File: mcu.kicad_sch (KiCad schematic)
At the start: 41 parts, among them J1 GPIO, J2 3v3/GND, Q1 MMBTA42, U1 STM32F103C8Tx, X1 SPI_DBG, X2 MTRBTN, X3 Bluetooth, X4 Buzzer, Y1 8MHz

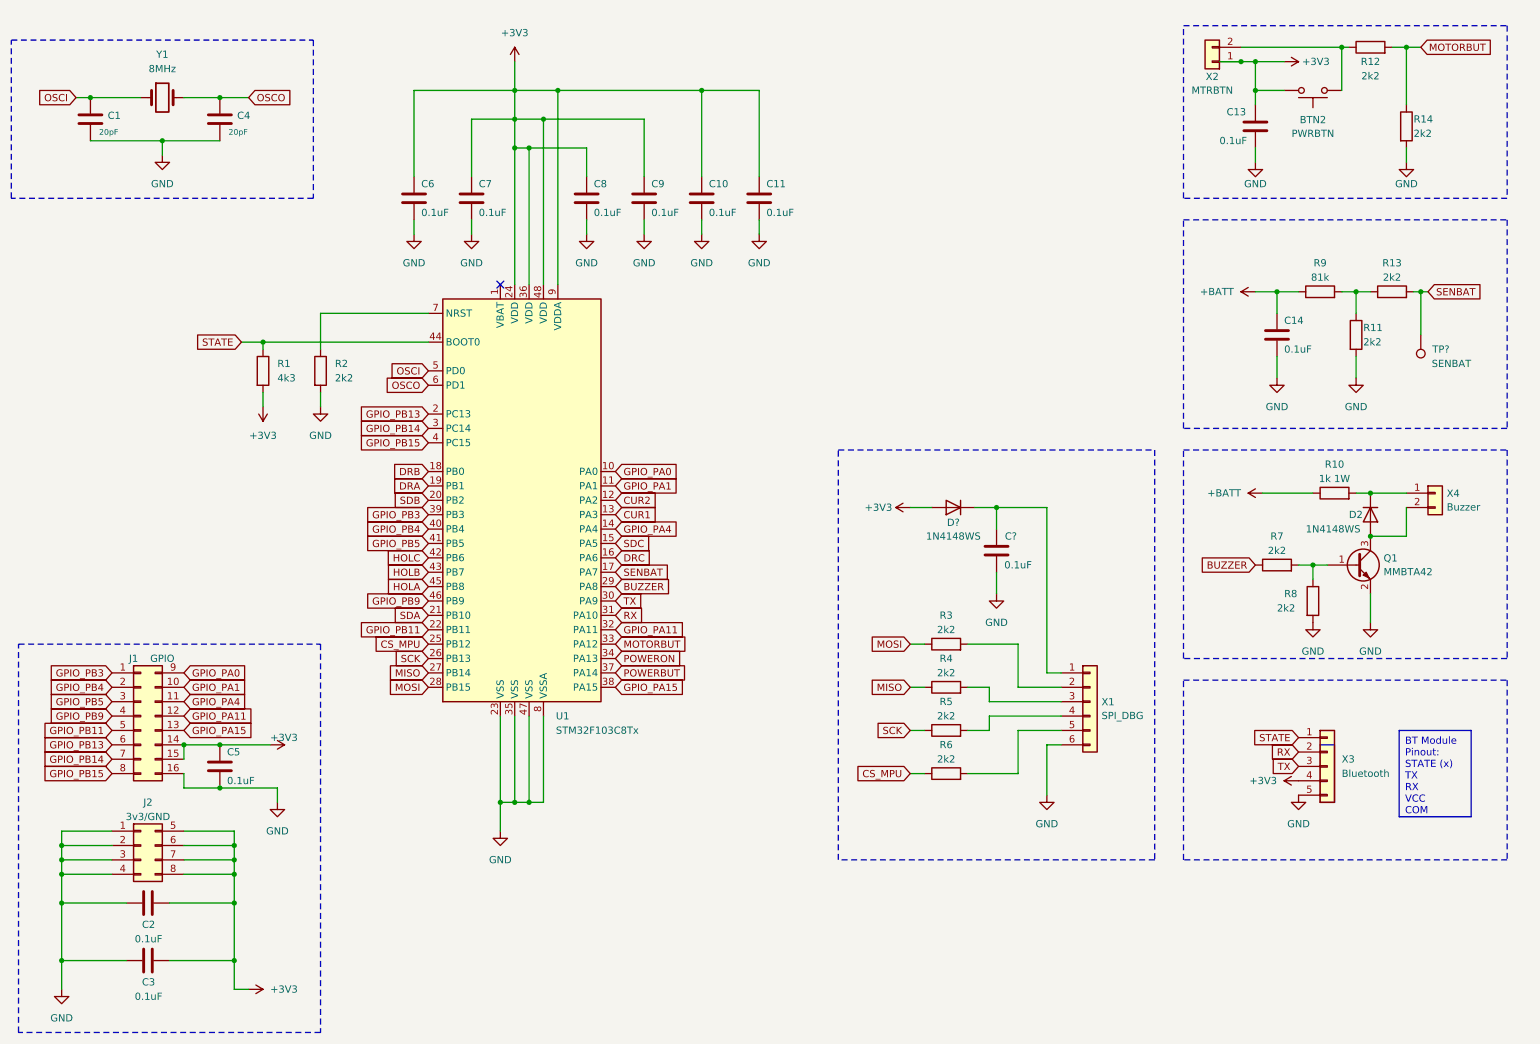
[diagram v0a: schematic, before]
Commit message: Minors, annotation
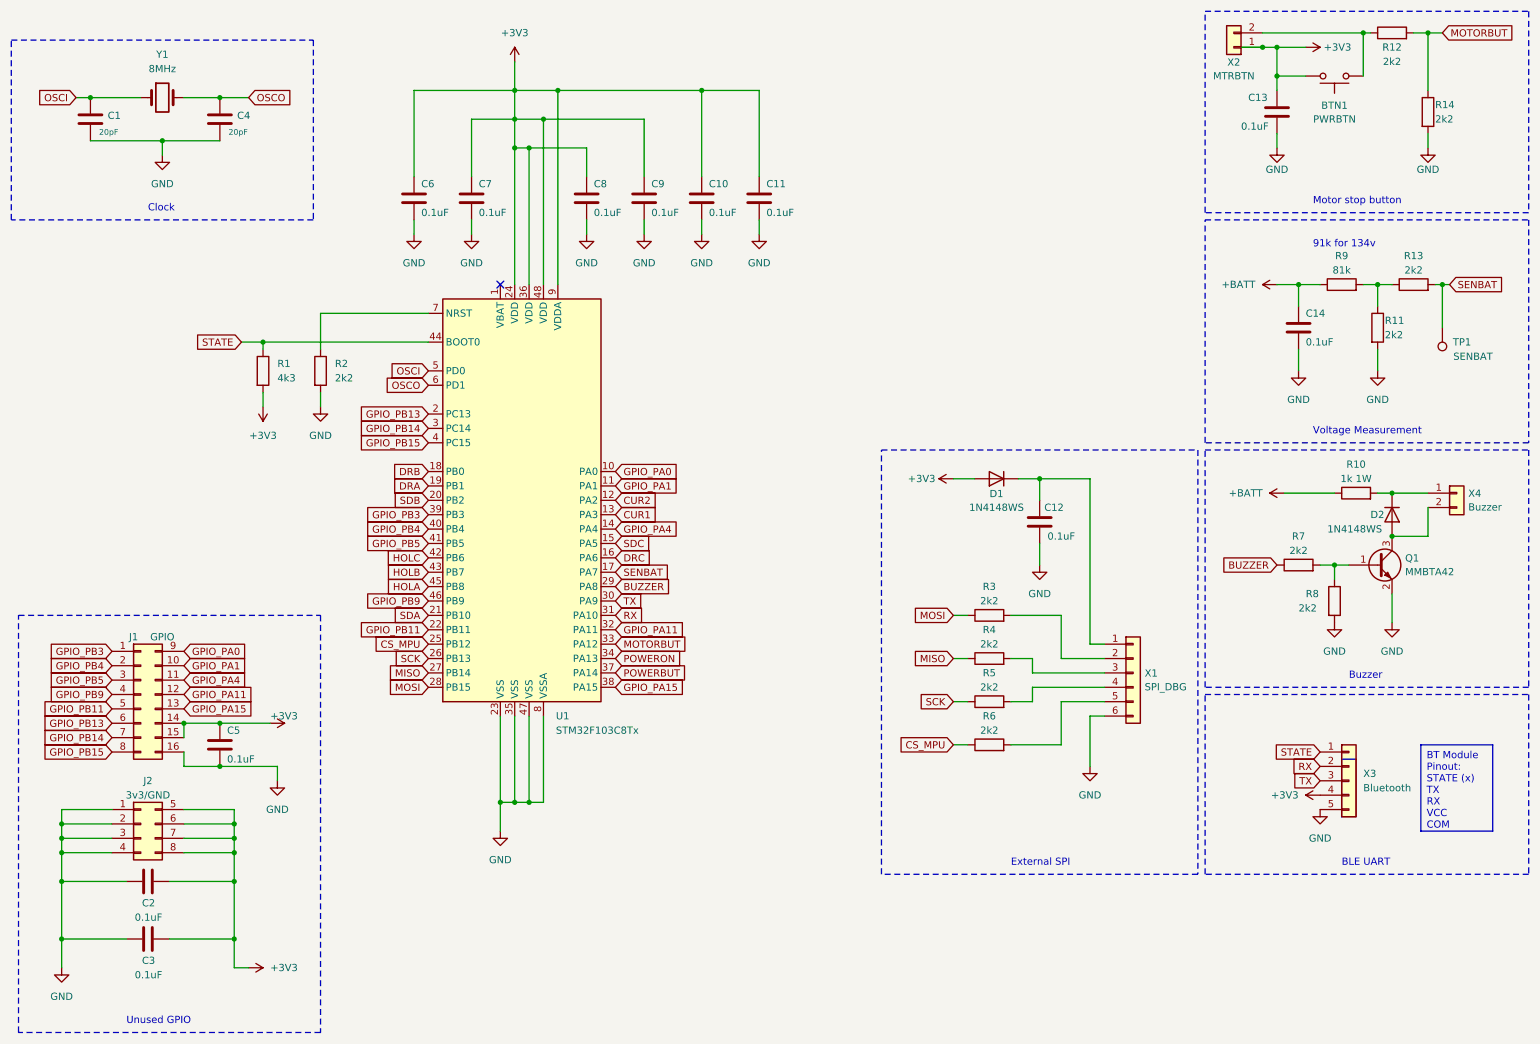
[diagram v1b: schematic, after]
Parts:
- gave numbers to parts that had none: 3
- renumbered BTN2 to BTN1
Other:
- note added: "91k for 134v"
- note added: "BLE UART"
- note added: "Buzzer"
- note added: "Clock"
- note added: "External SPI"
- note added: "Motor stop button"
- note added: "Unused GPIO"
- note added: "Voltage Measurement"
- title: (none) -> RedShift-117.6-LogicBoard-F103
- moved on the sheet: BTN1, C12, C13, C14, C2, C3, C5, D1, D2, J1, J2, Q1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
